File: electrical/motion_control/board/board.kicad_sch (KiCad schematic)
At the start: 2 parts, among them J101 5V_IN, U101 AMS1117-3.3

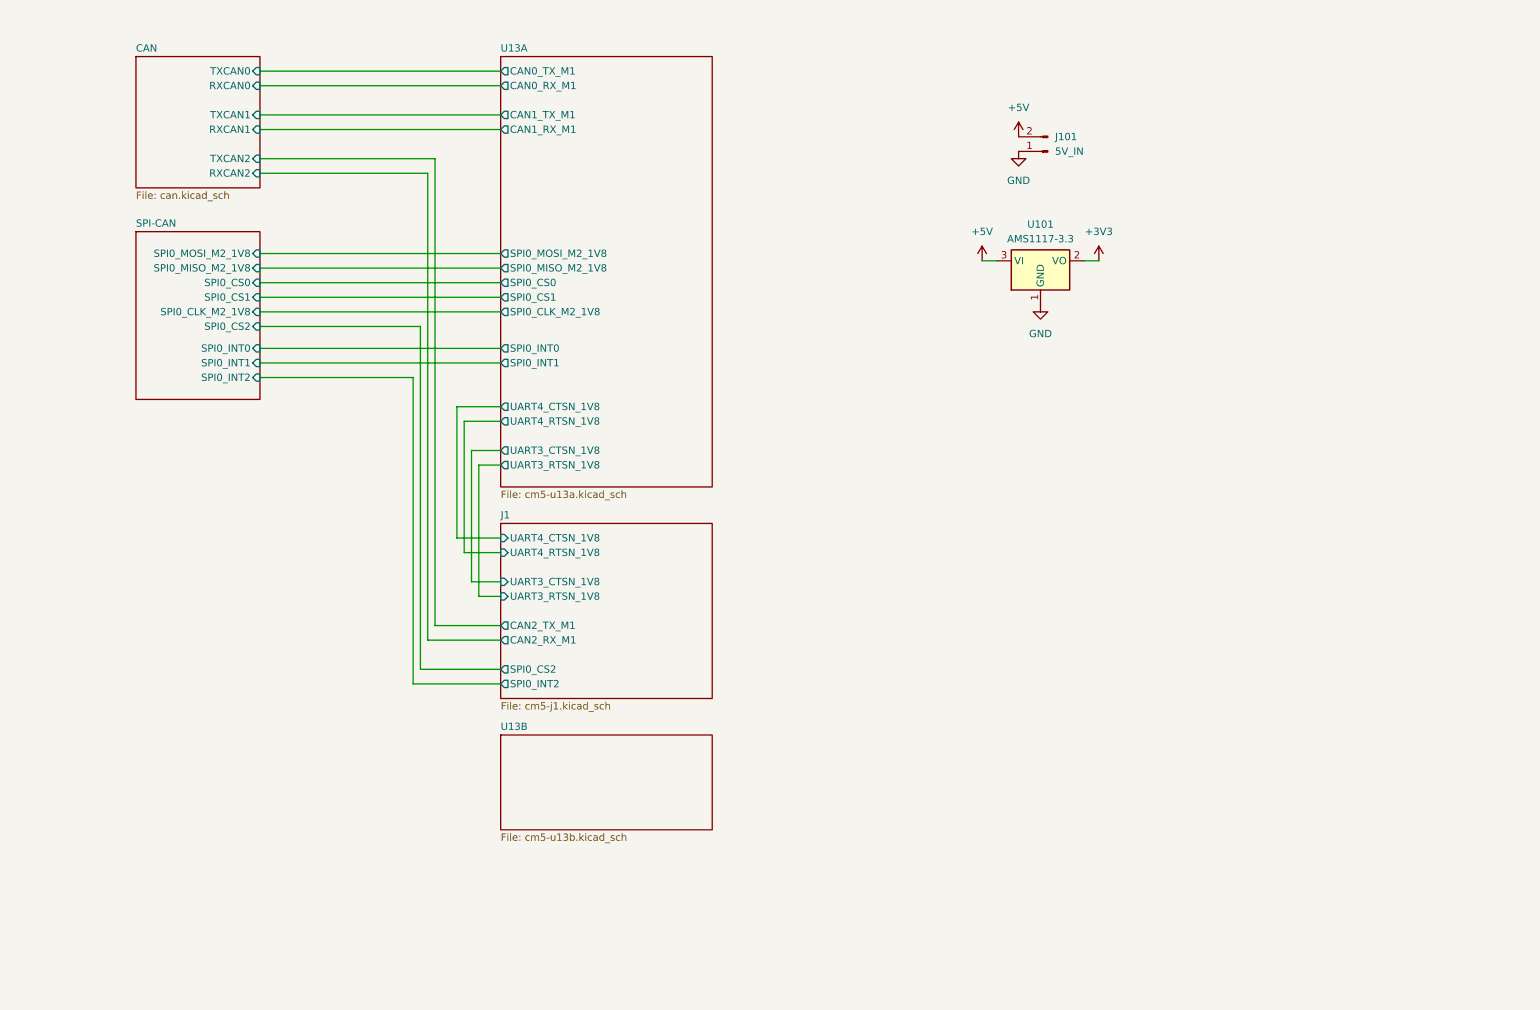
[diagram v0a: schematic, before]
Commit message: new boards, new device tree image
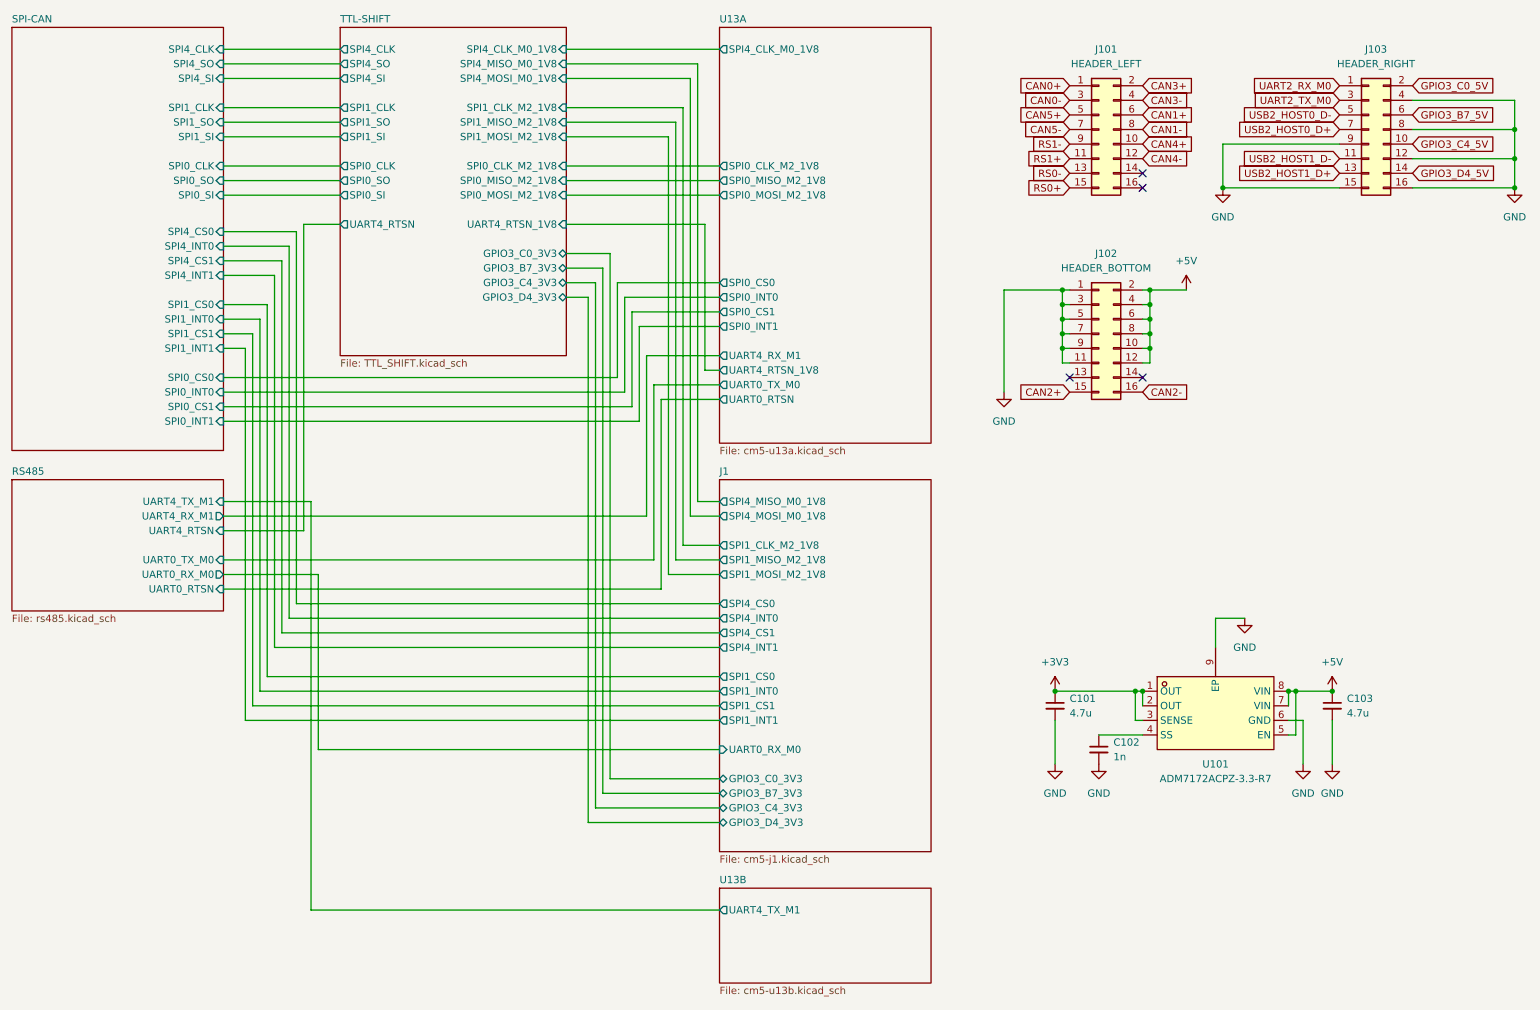
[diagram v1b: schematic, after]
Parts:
- removed J101: 5V_IN, Connector_AMASS:AMASS_XT30UPB-F_1x02_P5.0mm_Vertical, symbol Connector:Conn_01x02_Pin
- removed U101: AMS1117-3.3, Package_TO_SOT_SMD:SOT-223-3_TabPin2, symbol Regulator_Linear:AMS1117-3.3
- added C101, C103: 4.7u, Capacitor_SMD:C_0402_1005Metric, symbol Device:C_Small
- added C102: 1n, Capacitor_SMD:C_0402_1005Metric, symbol Device:C_Small
- added J101: HEADER_LEFT, Connector_PinHeader_2.54mm:PinHeader_2x08_P2.54mm_Vertical, symbol Connector_Generic:Conn_02x08_Odd_Even
- added J102: HEADER_BOTTOM, Connector_PinHeader_2.54mm:PinHeader_2x08_P2.54mm_Vertical, symbol Connector_Generic:Conn_02x08_Odd_Even
- added J103: HEADER_RIGHT, Connector_PinHeader_2.54mm:PinHeader_2x08_P2.54mm_Vertical, symbol Connector_Generic:Conn_02x08_Odd_Even
- added U101: ADM7172ACPZ-3.3-R7, lcsc_lib:DFN-8_L3.0-W3.0-P0.50-BL-EP, symbol lcsc_lib:ADM7172ACPZ-3.3-R7
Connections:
- net +3V3: now also C101.1, U101.1 (OUT), U101.2 (OUT), U101.3 (SENSE)
- net +5V: now also C103.1, J102.10 (Pin_10), J102.12 (Pin_12), J102.2 (Pin_2), J102.4 (Pin_4), J102.6 (Pin_6), J102.8 (Pin_8), U101.5 (EN), U101.7 (VIN), U101.8 (VIN)
- net GND: now also C101.2, C102.2, C103.2, J102.1 (Pin_1), J102.11 (Pin_11), J102.3 (Pin_3), J102.5 (Pin_5), J102.7 (Pin_7), J102.9 (Pin_9), J103.12 (Pin_12), J103.15 (Pin_15), J103.16 (Pin_16), J103.4 (Pin_4), J103.8 (Pin_8), J103.9 (Pin_9), U101.6 (GND), U101.9 (EP)
- new net: C102.1, U101.4 (SS)
- new net CAN0+: J101.1 (Pin_1)
- new net CAN0-: J101.3 (Pin_3)
- new net CAN1+: J101.6 (Pin_6)
- new net CAN1-: J101.8 (Pin_8)
- new net CAN2+: J102.15 (Pin_15)
- new net CAN2-: J102.16 (Pin_16)
- new net CAN3+: J101.2 (Pin_2)
- new net CAN3-: J101.4 (Pin_4)
- new net CAN4+: J101.10 (Pin_10)
- new net CAN4-: J101.12 (Pin_12)
- new net CAN5+: J101.5 (Pin_5)
- new net CAN5-: J101.7 (Pin_7)
- new net GPIO3_B7_5V: J103.6 (Pin_6)
- new net GPIO3_C0_5V: J103.2 (Pin_2)
- new net GPIO3_C4_5V: J103.10 (Pin_10)
- new net GPIO3_D4_5V: J103.14 (Pin_14)
- new net RS0+: J101.15 (Pin_15)
- new net RS0-: J101.13 (Pin_13)
- new net RS1+: J101.11 (Pin_11)
- new net RS1-: J101.9 (Pin_9)
- new net UART2_RX_M0: J103.1 (Pin_1)
- new net UART2_TX_M0: J103.3 (Pin_3)
- new net USB2_HOST0_D+: J103.7 (Pin_7)
- new net USB2_HOST0_D-: J103.5 (Pin_5)
- new net USB2_HOST1_D+: J103.13 (Pin_13)
- new net USB2_HOST1_D-: J103.11 (Pin_11)
- no-connect marks 0 -> 4
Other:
- removed sheet CAN
- added sheet RS485 (rs485.kicad_sch)
- added sheet TTL-SHIFT (TTL_SHIFT.kicad_sch)
- sheet J1 ports: added GPIO3_B7_3V3, GPIO3_C0_3V3, GPIO3_C4_3V3, GPIO3_D4_3V3, SPI1_CLK_M2_1V8, SPI1_CS0, SPI1_CS1, SPI1_INT0, SPI1_INT1, SPI1_MISO_M2_1V8, SPI1_MOSI_M2_1V8, SPI4_CS0, SPI4_CS1, SPI4_INT0, SPI4_INT1, SPI4_MISO_M0_1V8, SPI4_MOSI_M0_1V8, UART0_RX_M0; removed CAN2_RX_M1, CAN2_TX_M1, SPI0_CS2, SPI0_INT2, UART3_CTSN_1V8, UART3_RTSN_1V8, UART4_CTSN_1V8, UART4_RTSN_1V8
- sheet SPI-CAN ports: added SPI0_CLK, SPI0_SI, SPI0_SO, SPI1_CLK, SPI1_CS0, SPI1_CS1, SPI1_INT0, SPI1_INT1, SPI1_SI, SPI1_SO, SPI4_CLK, SPI4_CS0, SPI4_CS1, SPI4_INT0, SPI4_INT1, SPI4_SI, SPI4_SO; removed SPI0_CLK_M2_1V8, SPI0_CS2, SPI0_INT2, SPI0_MISO_M2_1V8, SPI0_MOSI_M2_1V8
- sheet U13A ports: added SPI4_CLK_M0_1V8, UART0_RTSN, UART0_TX_M0, UART4_RX_M1; removed CAN0_RX_M1, CAN0_TX_M1, CAN1_RX_M1, CAN1_TX_M1, UART3_CTSN_1V8, UART3_RTSN_1V8, UART4_CTSN_1V8
- sheet U13B ports: added UART4_TX_M1; removed none
